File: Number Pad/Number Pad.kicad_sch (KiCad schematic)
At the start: 42 parts, among them J1 Conn_01x19_Female, J2 Conn_01x19_Male

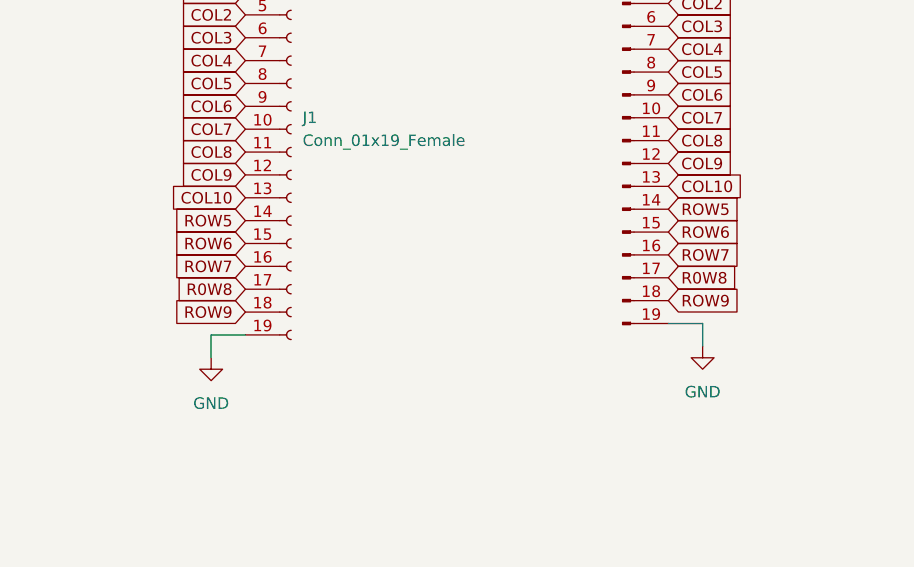
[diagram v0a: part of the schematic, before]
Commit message: Finished routing
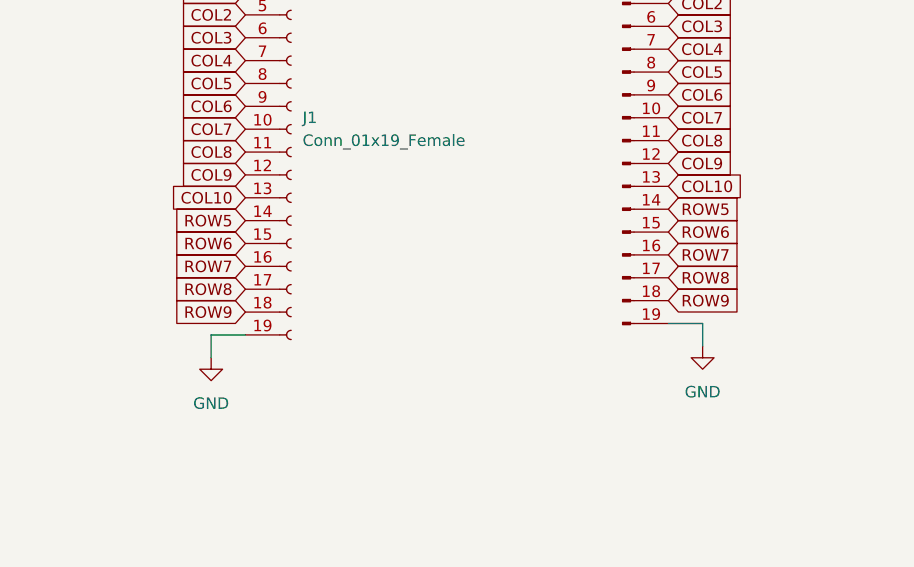
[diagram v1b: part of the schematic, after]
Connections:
- net R0W8 is gone; now on net ROW8: J1.17 (Pin_17), J2.17 (Pin_17)
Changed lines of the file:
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@@
     )
   )
-  (global_label "R0W8" (shape input) (at 189.23 107.95 180) (fields_autoplaced)
+  (global_label "ROW8" (shape input) (at 189.23 107.95 180) (fields_autoplaced)
     (effects (font (size 1.27 1.27)) (justify right))
-    (property "Intersheet References" "${INTERSHEET_REFS}" (id 0) (at 181.6764 107.8706 0)
+    (property "Intersheet References" "${INTERSHEET_REFS}" (id 0) (at 181.5555 107.8706 0)
       (effects (font (size 1.27 1.27)) (justify right) hide)
     )
@@
     )
   )
-  (global_label "R0W8" (shape input) (at 236.22 106.68 0) (fields_autoplaced)
+  (global_label "ROW8" (shape input) (at 236.22 106.68 0) (fields_autoplaced)
     (effects (font (size 1.27 1.27)) (justify left))
-    (property "Intersheet References" "${INTERSHEET_REFS}" (id 0) (at 243.7736 106.6006 0)
+    (property "Intersheet References" "${INTERSHEET_REFS}" (id 0) (at 243.8945 106.6006 0)
       (effects (font (size 1.27 1.27)) (justify left) hide)
     )
